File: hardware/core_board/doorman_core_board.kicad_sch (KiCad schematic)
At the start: 64 parts, among them J1 USB-C Connector, J10 VCC Test Pad, J11 TC BUS RX Test Pad, J12 Bus Voltage Test Pad, J2 Screw Terminals, J3 3V3 Test Pad, J4 Extension Board Connector, J5 Siedle BUS RX Test Pad, J6 BUS Test Pad, J7 BUS RX Test Pad, J8 TX Test Pad, J9 RX Test Pad, Q1 BC847BPN, Q2 BC817-40, Q3 IRLML0030, Q5 IRLML0030, Q6 BC847BPN, SW1 Button, SW2 Button, U2 AP63203WU, U3 GAQY252G3S, U4 ESP32-S3-MINI-1

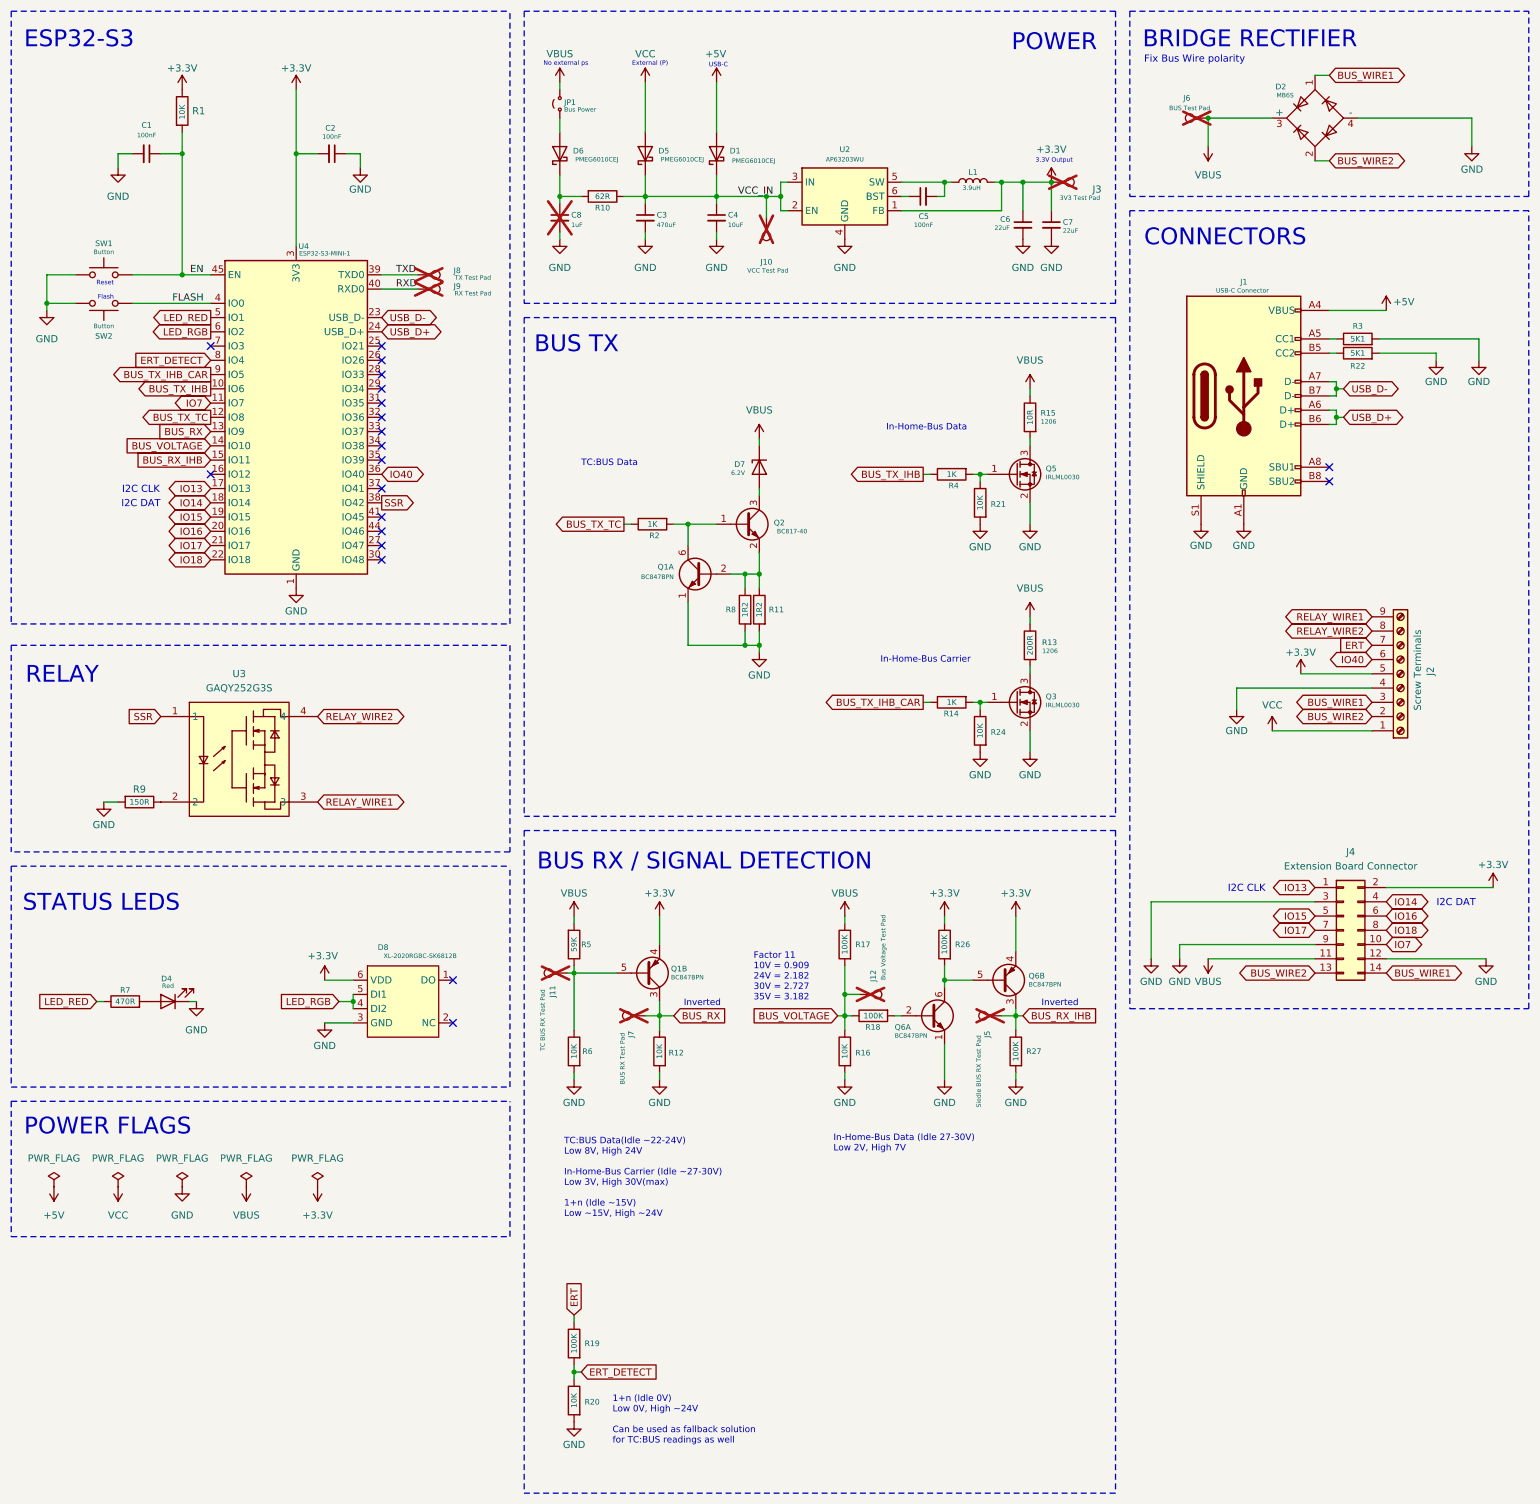
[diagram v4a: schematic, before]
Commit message: chore: Update pcb files 2.2.0
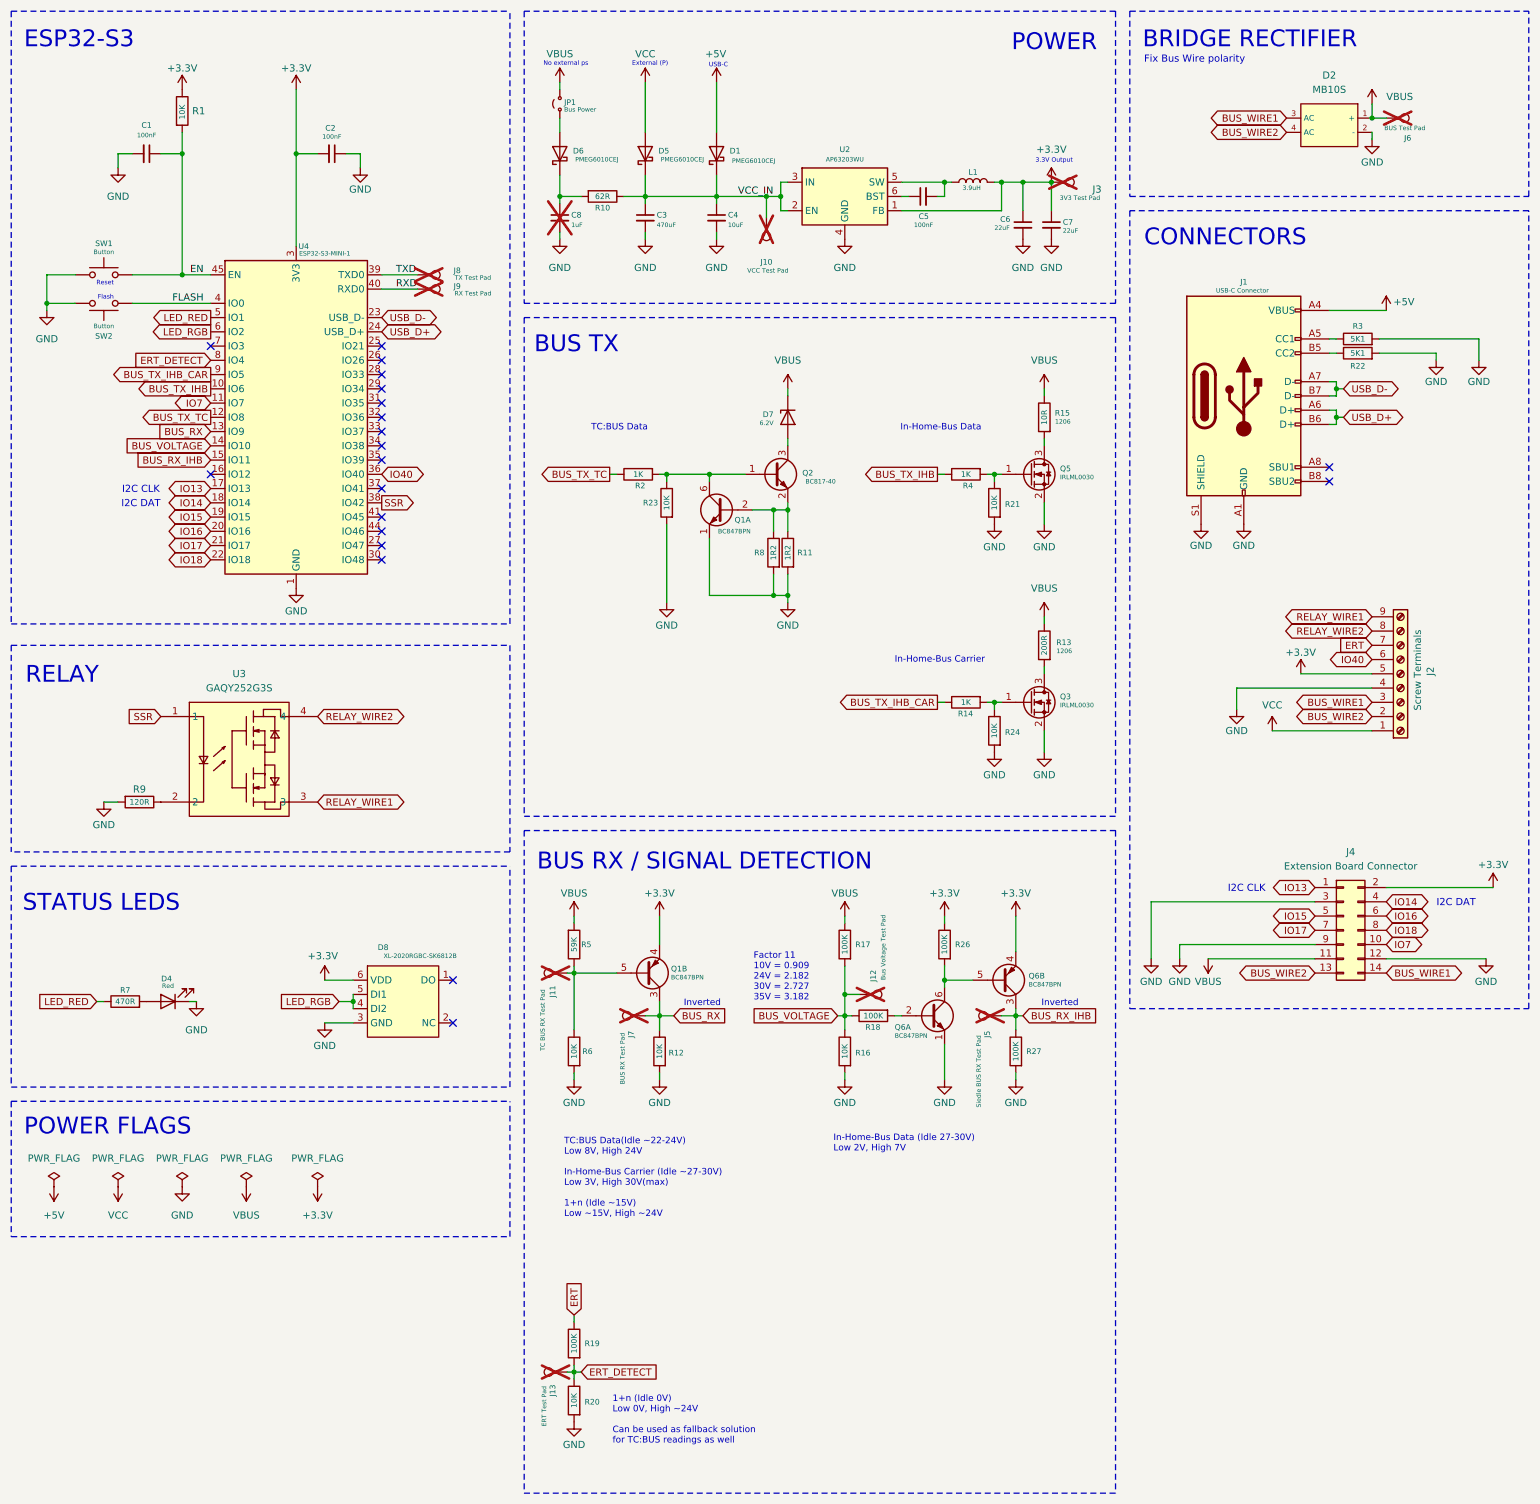
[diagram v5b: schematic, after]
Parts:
- removed D2: MB6S, Package_TO_SOT_SMD:TO-269AA, symbol Diode_Bridge:MB6S
- added D2: MB10S, Package_TO_SOT_SMD:TO-269AA, symbol PCM_JLCPCB-Diode-Packages:Bridge Rectifier, MB10S
- added J13: ERT Test Pad, TestPoint:TestPoint_Pad_D1.0mm, symbol Connector:TestPoint
- added R23: 10K, Resistor_SMD:R_0603_1608Metric, symbol Device:R
- Q3, Q5: LCSC C67272 -> C6285737; MPN IRLML0030TRPBF -> IRLML0030TRPBF-HXY
- R9: value 150R -> 120R; LCSC C25082 -> C25079; MPN 0402WGF1500TCE -> 0402WGF1200TCE
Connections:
- net BUS_WIRE1: now also D2.3 (AC)
- net BUS_WIRE2: now also D2.4 (AC)
- net ERT_DETECT: now also J13.1
- net GND: now also D2.2 (-), R23.2
- net VBUS: now also D2.1 (+)
- net at Q1.6 (C1), Q2.1 (B), R2.2: now also R23.1
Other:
- moved on the sheet: D7, J6, Q1A, Q2, Q3, Q5, R11, R13, R14, R15, R2, R21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
